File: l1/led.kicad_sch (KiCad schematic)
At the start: 30 parts

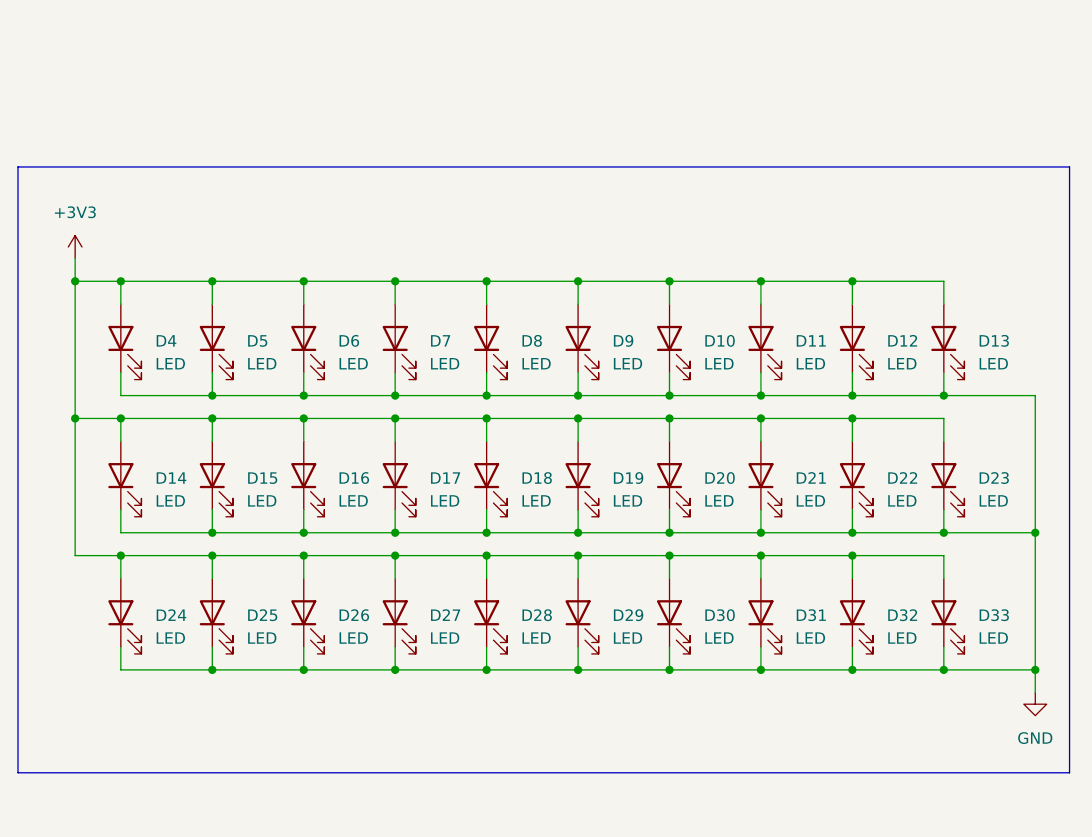
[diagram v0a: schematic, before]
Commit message: rough ideation
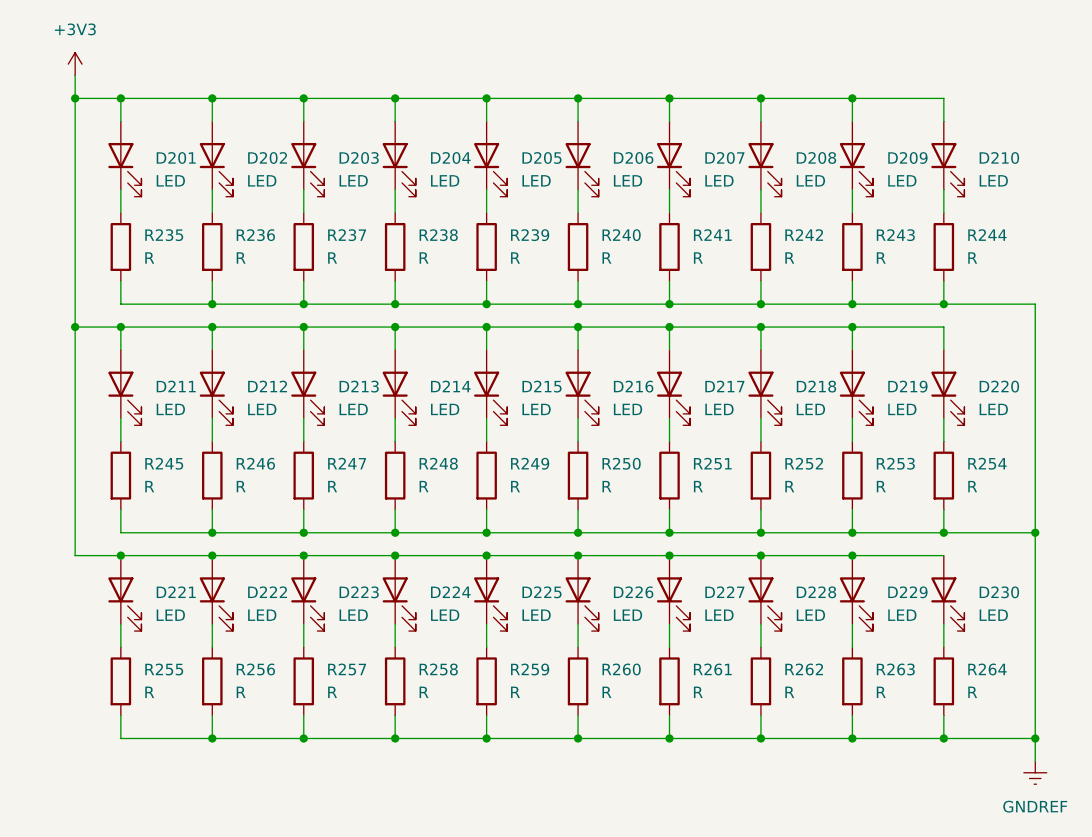
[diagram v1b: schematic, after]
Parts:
- removed D10, D11, D12, D13, D14, D15, D16, D17, D18, D19, D20, D21, D22, D23, D24, D25, D26, D27, D28, D29, D30, D31, D32, D33, D4, D5, D6, D7, D8, D9: LED, Library:led2835, symbol Device:LED
- added D201, D202, D203, D204, D205, D206, D207, D208, D209, D210, D211, D212, D213, D214, D215, D216, D217, D218, D219, D220, D221, D222, D223, D224, D225, D226, D227, D228, D229, D230: LED, Library:led2835, symbol Device:LED
- added R235, R236, R237, R238, R239, R240, R241, R242, R243, R244, R245, R246, R247, R248, R249, R250, R251, R252, R253, R254, R255, R256, R257, R258, R259, R260, R261, R262, R263, R264: R, Library:res0603, symbol Device:R
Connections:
- net +3V3: now also D201.2 (A), D202.2 (A), D203.2 (A), D204.2 (A), D205.2 (A), D206.2 (A), D207.2 (A), D208.2 (A), D209.2 (A), D210.2 (A), D211.2 (A), D212.2 (A), D213.2 (A), D214.2 (A), D215.2 (A), D216.2 (A), D217.2 (A), D218.2 (A), D219.2 (A), D220.2 (A), D221.2 (A), D222.2 (A), D223.2 (A), D224.2 (A), D225.2 (A), D226.2 (A), D227.2 (A), D228.2 (A), D229.2 (A), D230.2 (A)
- new net: D212.1 (K), R246.1
- new net: D229.1 (K), R263.1
- new net: D215.1 (K), R249.1
- new net: D209.1 (K), R243.1
- new net: D202.1 (K), R236.1
- new net: D221.1 (K), R255.1
- new net: D218.1 (K), R252.1
- new net: D230.1 (K), R264.1
- new net: D216.1 (K), R250.1
- new net: D214.1 (K), R248.1
- new net: D225.1 (K), R259.1
- new net: D207.1 (K), R241.1
- new net: D226.1 (K), R260.1
- new net: D224.1 (K), R258.1
- new net: D223.1 (K), R257.1
- new net: D204.1 (K), R238.1
- new net: D206.1 (K), R240.1
- new net: D211.1 (K), R245.1
- new net: D217.1 (K), R251.1
- new net: D227.1 (K), R261.1
- new net: D201.1 (K), R235.1
- new net: D219.1 (K), R253.1
- new net: D222.1 (K), R256.1
- new net: D210.1 (K), R244.1
- new net: D220.1 (K), R254.1
- new net: D208.1 (K), R242.1
- new net: D203.1 (K), R237.1
- new net: D213.1 (K), R247.1
- new net: D205.1 (K), R239.1
- new net: D228.1 (K), R262.1
- new net GNDREF: R235.2, R236.2, R237.2, R238.2, R239.2, R240.2, R241.2, R242.2, R243.2, R244.2, R245.2, R246.2, R247.2, R248.2, R249.2, R250.2, R251.2, R252.2, R253.2, R254.2, R255.2, R256.2, R257.2, R258.2, R259.2, R260.2, R261.2, R262.2, R263.2, R264.2

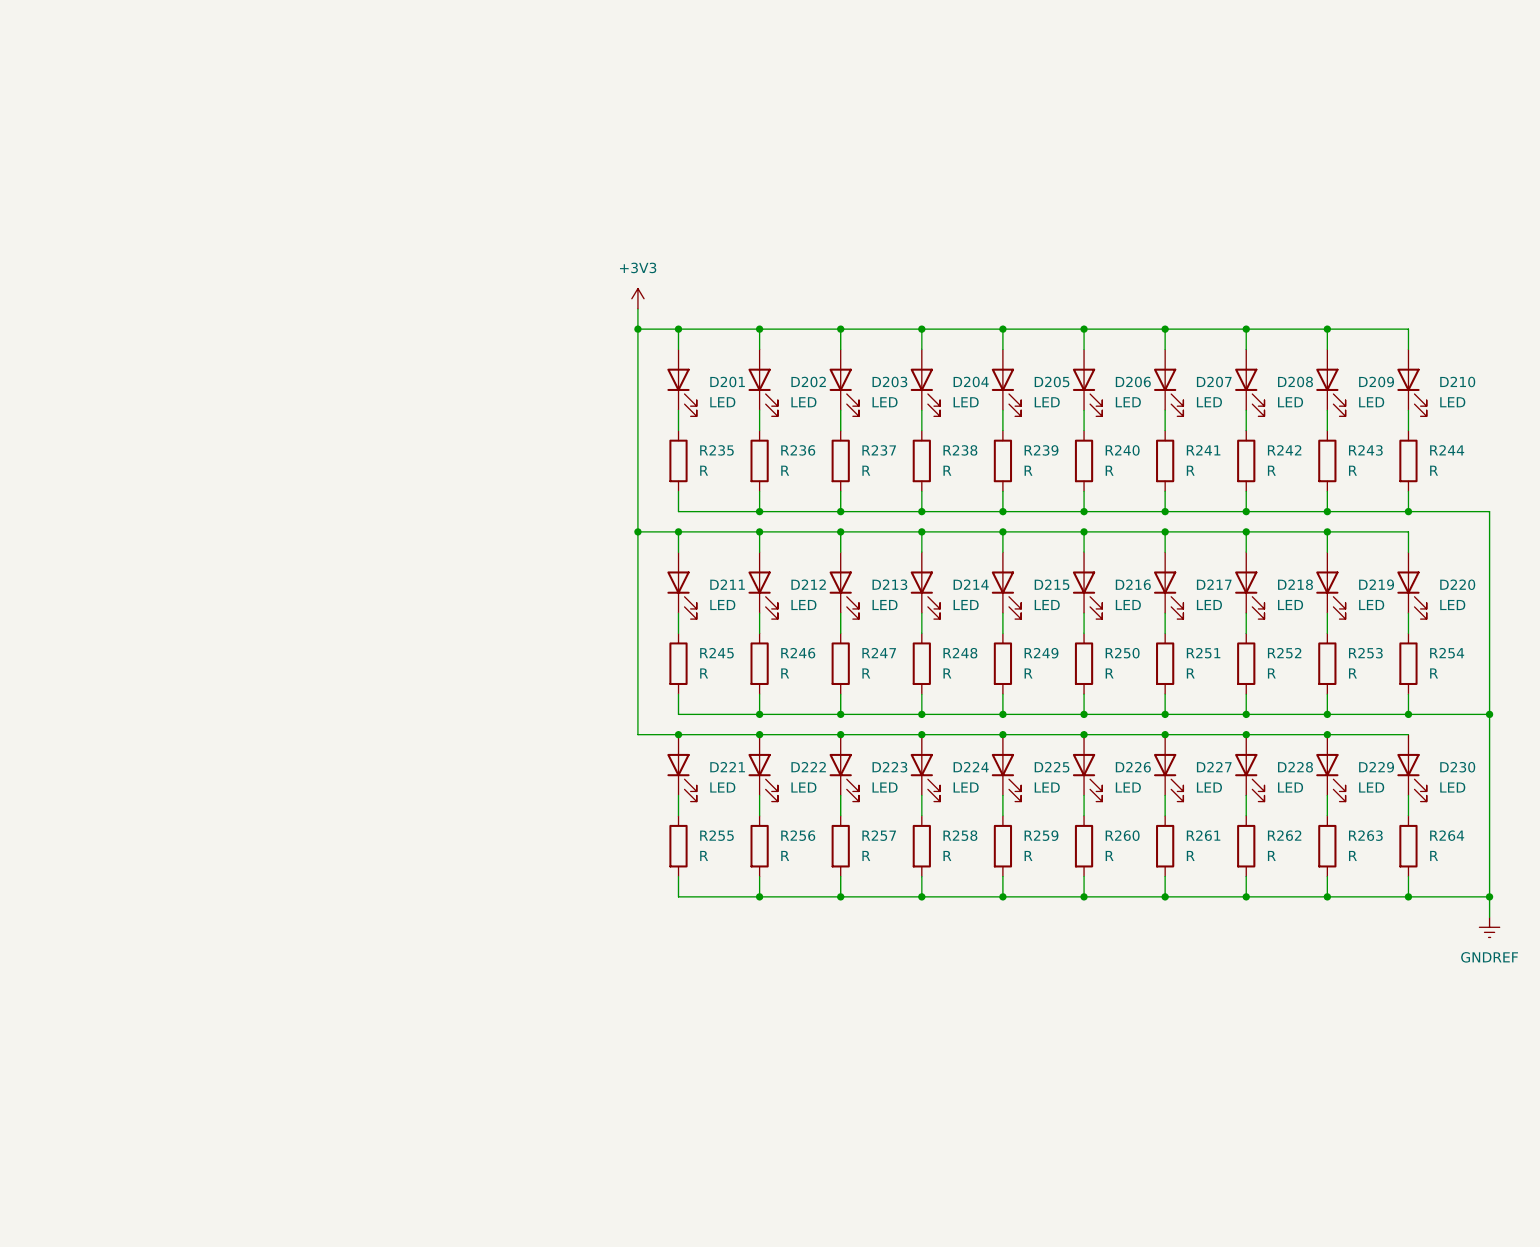
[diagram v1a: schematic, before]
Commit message: 死
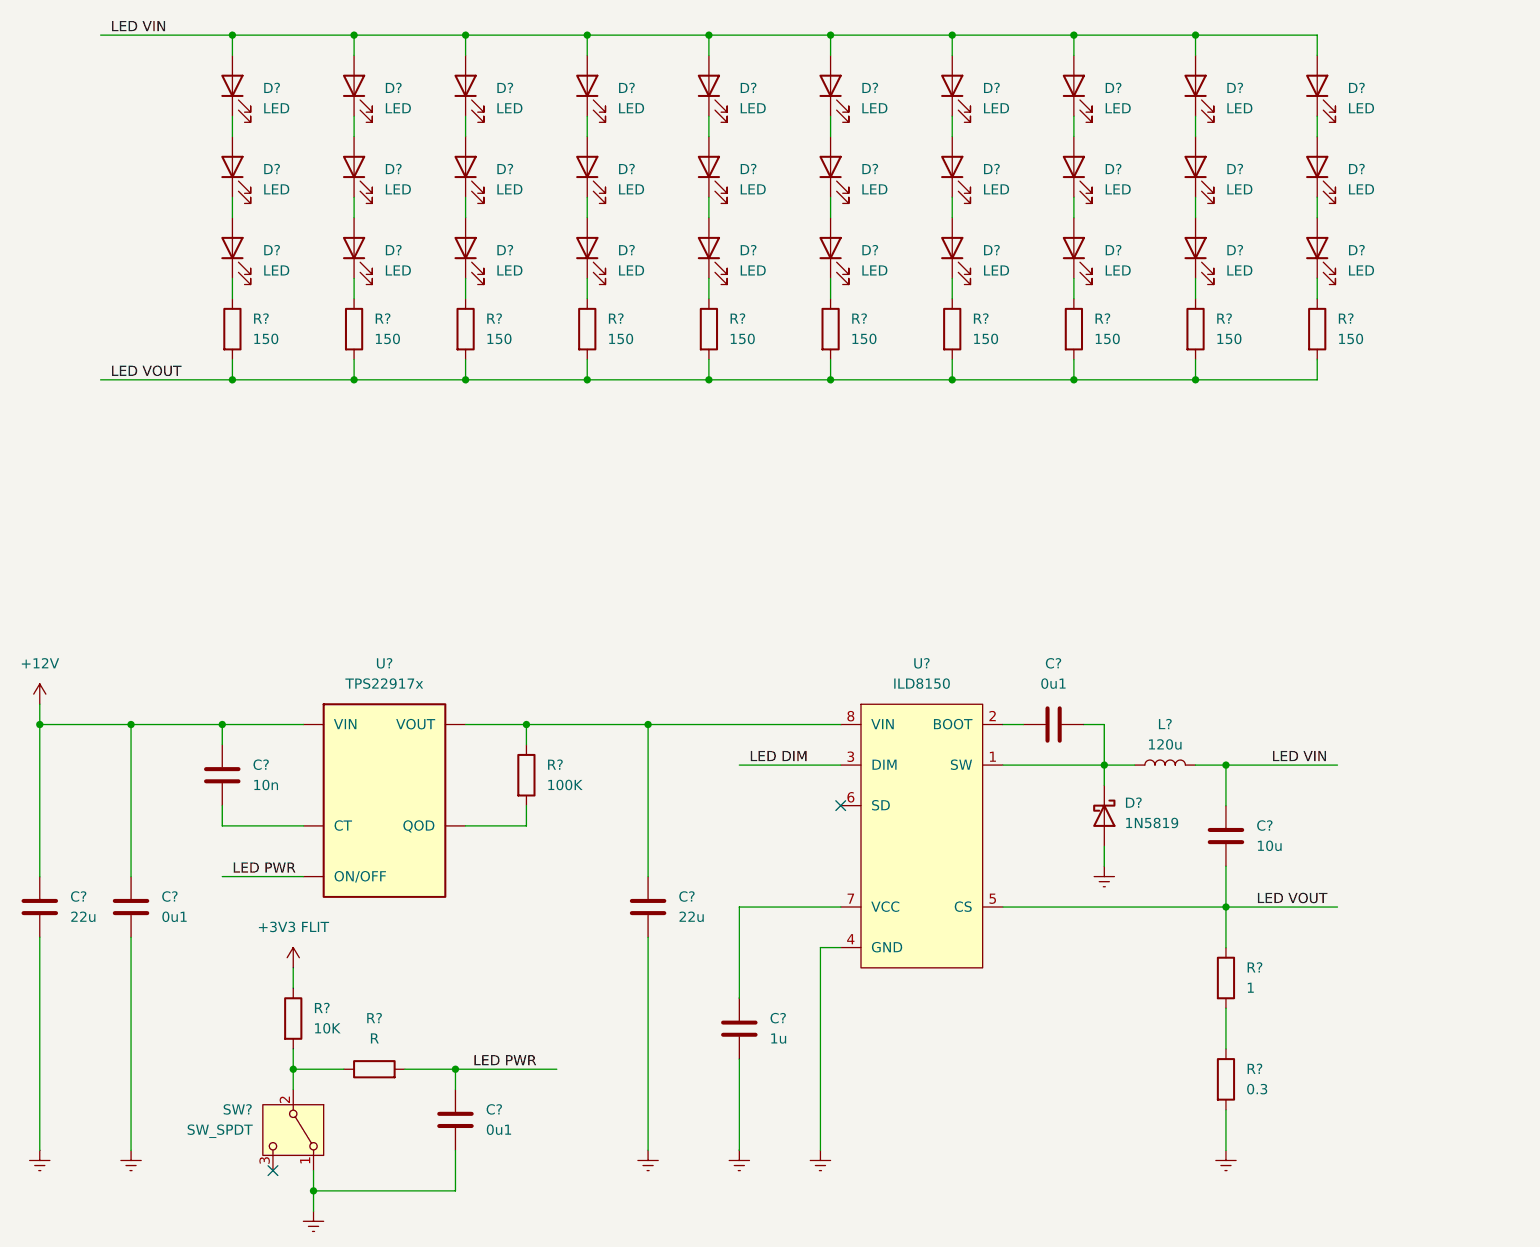
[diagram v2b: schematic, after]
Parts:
- removed D201, D202, D203, D204, D205, D206, D207, D208, D209, D210, D211, D212, D213, D214, D215, D216, D217, D218, D219, D220, D221, D222, D223, D224, D225, D226, D227, D228, D229, D230: LED, Library:led2835, symbol Device:LED
- removed R235, R236, R237, R238, R239, R240, R241, R242, R243, R244, R245, R246, R247, R248, R249, R250, R251, R252, R253, R254, R255, R256, R257, R258, R259, R260, R261, R262, R263, R264: R, Library:res0603, symbol Device:R
- added C? (x2): 22u, symbol Device:C
- added C? (x3): 0u1, symbol Device:C
- added C?: 10n, symbol Device:C
- added C?: 1u, symbol Device:C
- added C?: 10u, symbol Device:C
- added D? (x30): LED, Library:led2835, symbol Device:LED
- added D?: 1N5819, symbol Device:D_Schottky
- added L?: 120u, symbol Device:L
- added R?: 10K, symbol Device:R
- added R?: 1, symbol Device:R
- added R?: R, symbol Device:R
- added R? (x10): 150, Library:res0603, symbol Device:R
- added R?: 100K, symbol Device:R
- added R?: 0.3, symbol Device:R
- added SW?: SW_SPDT, symbol Switch:SW_SPDT
- added U?: TPS22917x, symbol vincent:TPS22917x
- added U?: ILD8150, symbol vincent:ILD8150
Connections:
- new net: D?.1 (K), D?.2 (A) (x20)
- new net: D?.1 (K), R?.1 (x10)
- new net: R?.1, R?.2, SW?.2 (B)
- new net: R?.1, R?.2
- new net: C?.1, R?.1, U?. (VOUT), U?.8 (VIN)
- new net: C?.2, D?.1 (K), L?.1, U?.1 (SW)
- new net: C?.1, U?.2 (BOOT)
- new net: C?.2, U?. (VOUT)
- new net: R?.2, U?. (VOUT)
- new net: C?.1, U?.7 (VCC)
- new net +12V: C?.1, C?.1, C?.1, U?. (VOUT)
- new net +3V3 FLIT: R?.1
- new net EP: C?.2, C?.2, C?.2, C?.2, C?.2, D?.2 (A), R?.2, SW?.1 (A), U?.4 (GND), U?.9 (EP)
- new net LED DIM: U?.3 (DIM)
- new net LED PWR: C?.1, R?.2, U?. (VOUT)
- new net LED VIN: C?.1, D?.2 (A), D?.2 (A), D?.2 (A), D?.2 (A), D?.2 (A), D?.2 (A), D?.2 (A), D?.2 (A), D?.2 (A), D?.2 (A), L?.2
- new net LED VOUT: C?.2, R?.1, R?.2, R?.2, R?.2, R?.2, R?.2, R?.2, R?.2, R?.2, R?.2, R?.2, U?.5 (CS)
- no-connect marks 0 -> 2
